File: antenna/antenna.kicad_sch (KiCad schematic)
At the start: 24 parts, among them J1 Conn_01x05_Pin, J2 Conn_01x05_Pin, J3 Conn_01x05_Pin, J5 USB_C_Receptacle, SW1 SW_Push, SW2 SW_Push, U1 ESP32-C3-WROOM-02, U2 AMS1117-3.3

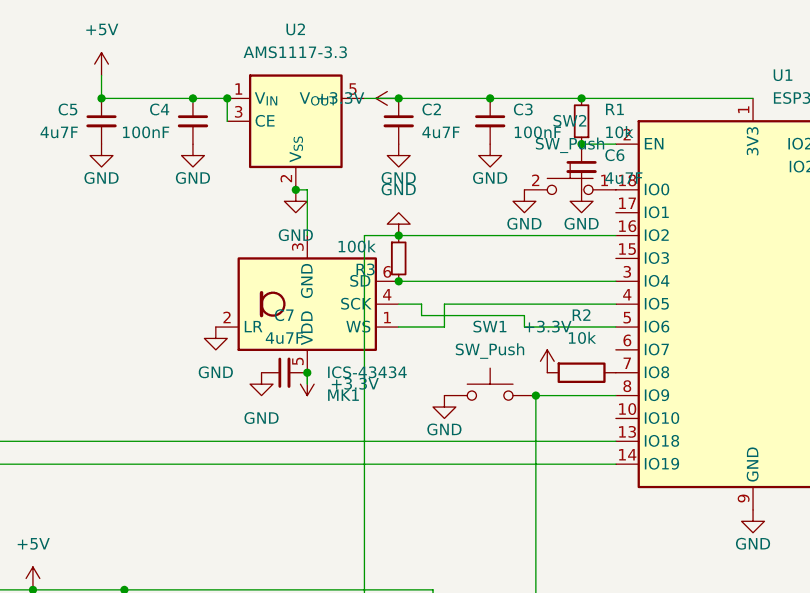
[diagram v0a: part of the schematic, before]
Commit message: url-update and some bla
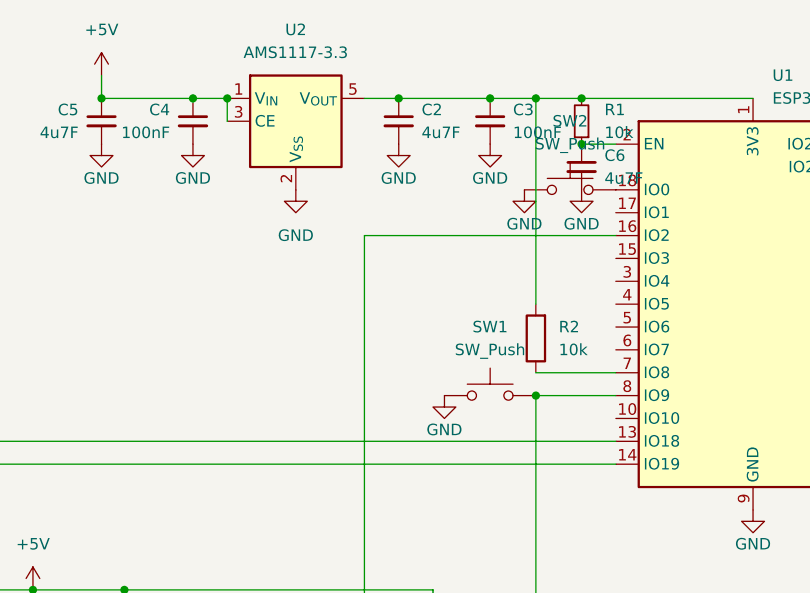
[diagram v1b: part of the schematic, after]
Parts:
- removed C7: 4u7F, Capacitor_SMD:C_0805_2012Metric_Pad1.18x1.45mm_HandSolder, symbol Device:C_Small
- removed MK1: ICS-43434, Sensor_Audio:InvenSense_ICS-43434-6_3.5x2.65mm, symbol Sensor_Audio:ICS-43434
- removed R3: 100k, Resistor_SMD:R_0805_2012Metric_Pad1.20x1.40mm_HandSolder, symbol Device:R_Small
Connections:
- net GND: now also SW2.1; no longer D1.2 (DIN), J1.3 (Pin_3), SW2.2, U1.16 (IO2)
- net at U1.18 (IO0): now also SW2.2; no longer SW2.1
- net +3.3V: no longer names the net of C2.1, C3.1, R1.2, R2.2, U1.1 (3V3), U2.5 (V_{OUT})
- new net: D1.2 (DIN), J1.3 (Pin_3), U1.16 (IO2)
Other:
- moved on the sheet: R2
